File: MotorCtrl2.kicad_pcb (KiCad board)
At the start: 2 copper layers, 38.1 x 50 mm, 12 parts, among them J1 Conn_01x02_Female, J2 Conn_01x02_Female, J3 Conn_01x02_Female, Q1 BS108, Q2 IRLB8721PBF

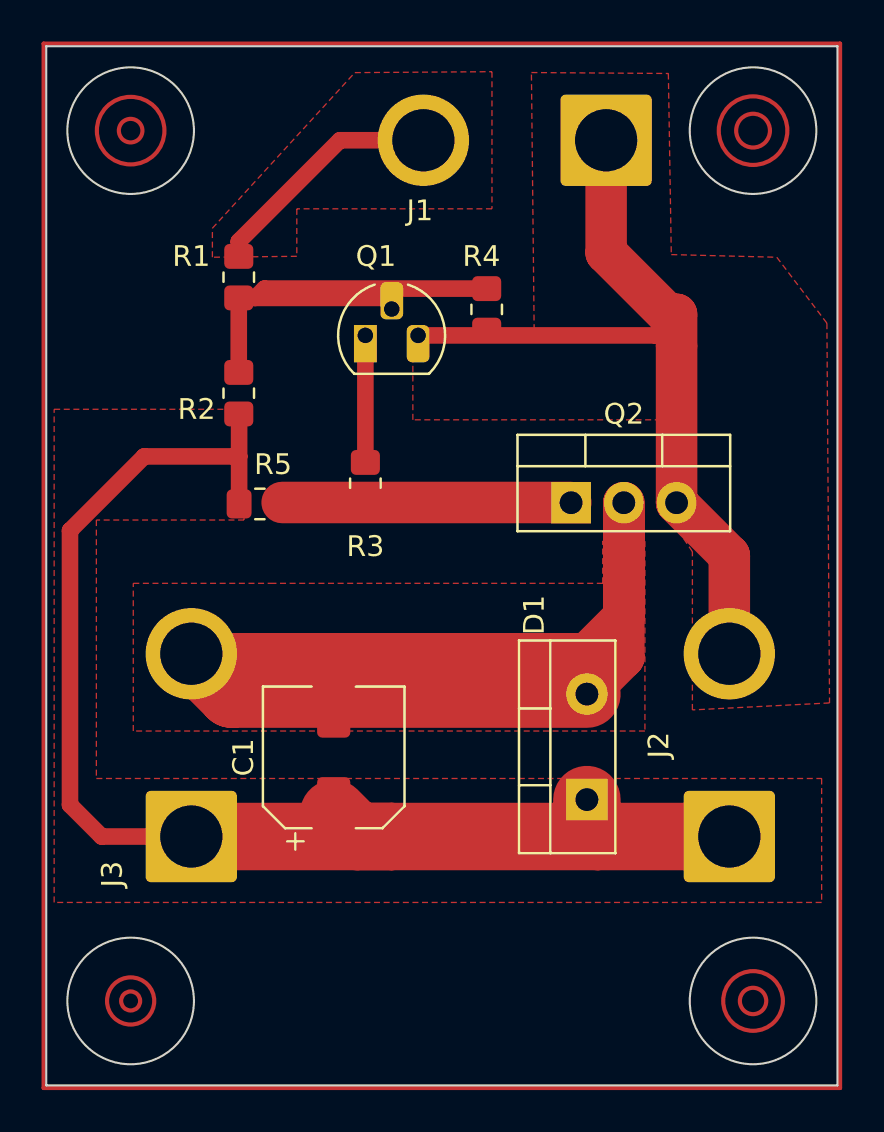
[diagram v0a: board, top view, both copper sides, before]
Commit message: .
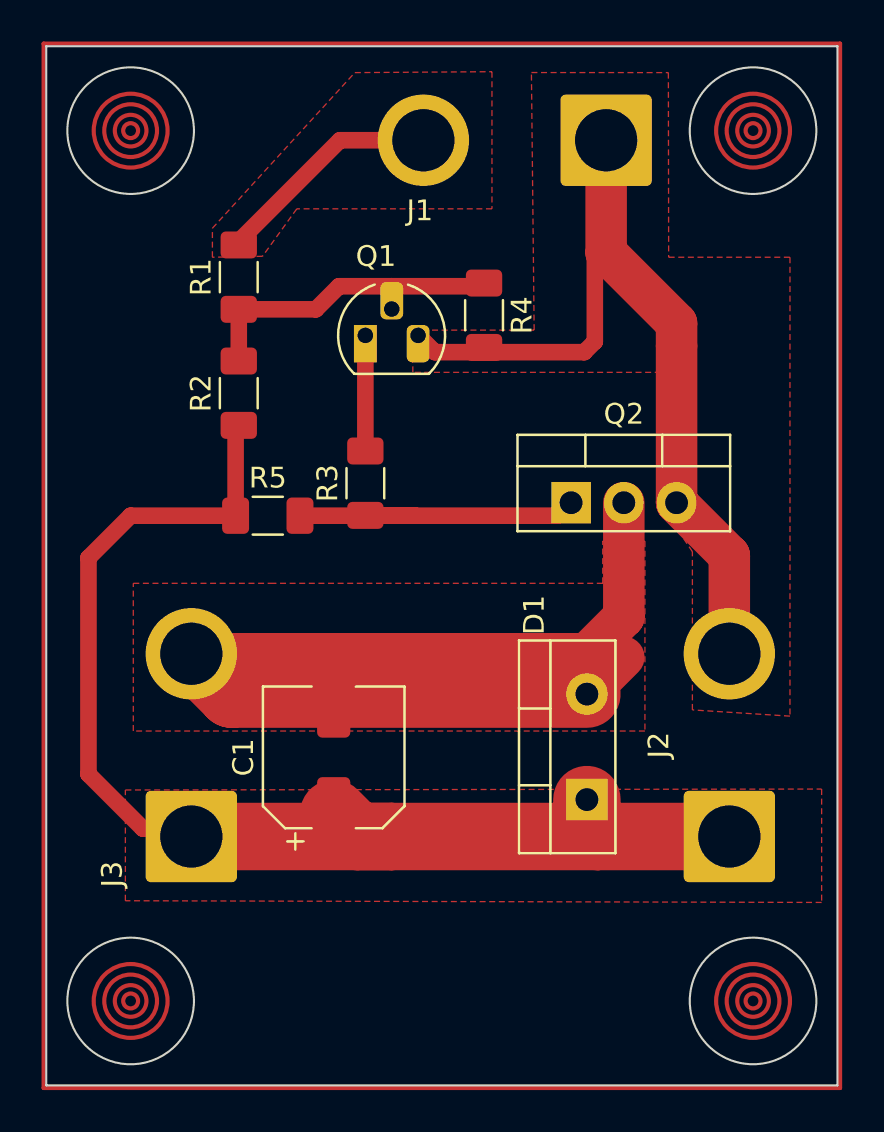
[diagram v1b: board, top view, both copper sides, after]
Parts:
- R1, R2, R3, R4, R5: footprint Resistor_SMD:R_0805_2012Metric_Pad1.20x1.40mm_HandSolder -> Resistor_SMD:R_1206_3216Metric_Pad1.30x1.75mm_HandSolder
- moved R5 0.68 mm to (11.2, 269.0)
- moved R4 0.31 mm to (21.6, 259.3)
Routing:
- net Net-(C1-Pad2): track 56.9 -> 49.4 mm
- net Net-(Q1-Pad2): track 21.8 -> 16.1 mm
- net +12V: track 64.8 -> 59.6 mm
- net GND: track 41.0 -> 43.8 mm
- net Net-(Q2-Pad1): track 14.1 -> 15.8 mm
- net Net-(Q1-Pad1): track 6.12 -> 5.57 mm
- net Net-(J1-Pad2): track 11.6 -> 11.1 mm
